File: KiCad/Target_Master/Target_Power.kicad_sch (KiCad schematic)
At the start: 8 parts, among them SW1 SW_SPST, U1 AMS1117-5

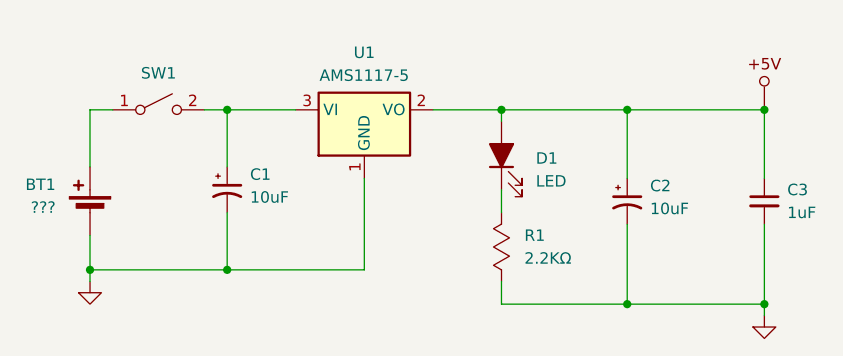
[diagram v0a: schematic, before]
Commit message: Finalized schematics
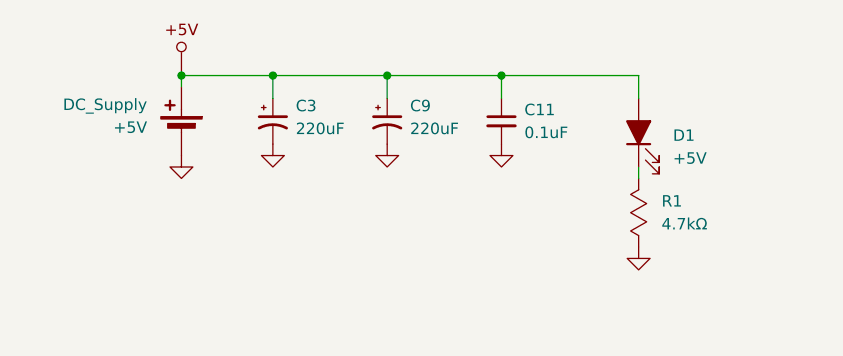
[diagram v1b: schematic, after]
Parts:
- removed BT1: ???, symbol Device:Battery_Cell
- removed C1, C2: 10uF, Capacitor_SMD:C_0805_2012Metric_Pad1.18x1.45mm_HandSolder, symbol Device:C_Polarized_Small_US
- removed C3: 1uF, Capacitor_SMD:C_0805_2012Metric_Pad1.18x1.45mm_HandSolder, symbol Device:C_Small
- removed SW1: SW_SPST, symbol Switch:SW_SPST
- removed U1: AMS1117-5, Package_TO_SOT_SMD:SOT-223-3_TabPin2, symbol Regulator_Linear:AMS1117-3.3
- added C11: 0.1uF, symbol Device:C_Small
- added C3, C9: 220uF, symbol Device:C_Polarized_Small_US
- added DC_Supply: +5V, symbol Device:Battery_Cell
- D1: value LED -> +5V; footprint LED_SMD:LED_0805_2012Metric_Pad1.15x1.40mm_HandSolder -> (none)
- R1: value 2.2KΩ -> 4.7kΩ; footprint Resistor_SMD:R_0805_2012Metric_Pad1.20x1.40mm_HandSolder -> (none)
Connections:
- net +5V: now also C11.1, C3.1, C9.1, DC_Supply.1 (+)
- net GND: now reaches R1.1
- net GND: now also C11.2, C3.2, C9.2, DC_Supply.2 (-)
